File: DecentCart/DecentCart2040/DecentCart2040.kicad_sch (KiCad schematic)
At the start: 75 parts, among them J1 Micro_SD_Card, J2 Conn_02x15_Row_Letter_First, J3 SM03B-SRSS-TB, J7 Conn_01x04, J8 USB_B_Micro, J9 SM03B-SRSS-TB, Q2 DMG2305UX, SW2 SW_TACTILE, SW3 SW_TACTILE, U1 SN74LVC8T245, U2 SN74LVC8T245, U3 ATtiny1616-M, U4 NCP1117-3.3, U5 SN74LVC8T245, U6 SN74AVC4T245PW, U7 RP2040, U9 W25Q128JVS, X1 12MHz

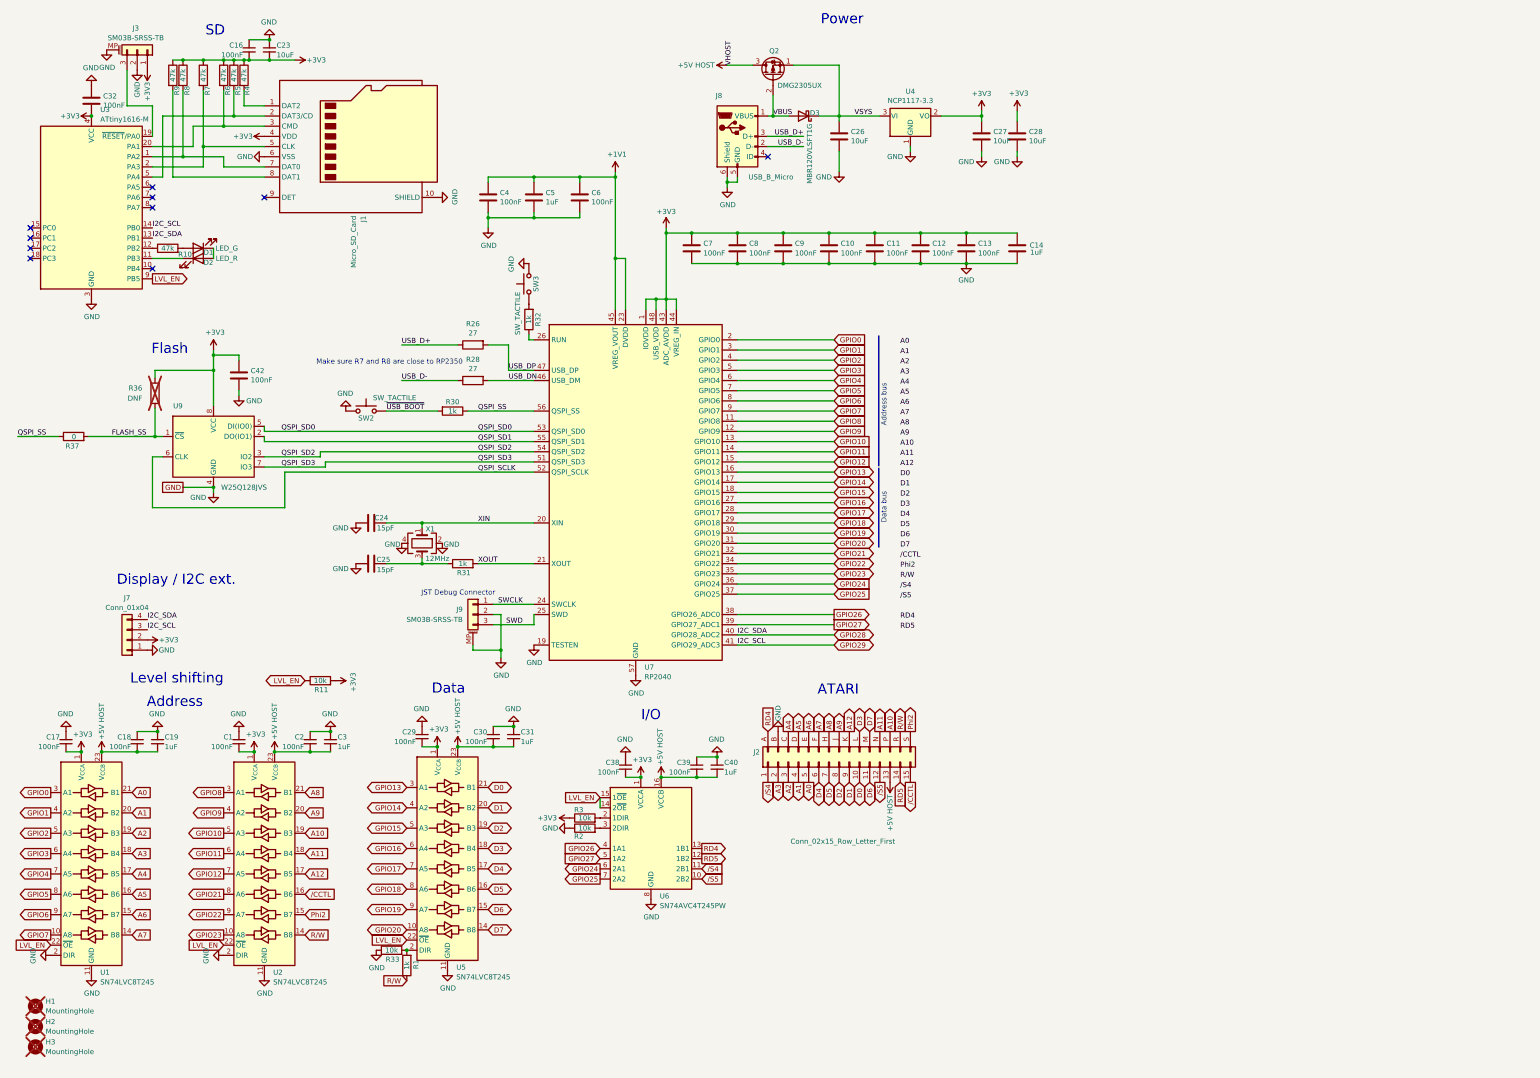
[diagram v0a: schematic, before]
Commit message: DecentCart2040 rev. 1.1
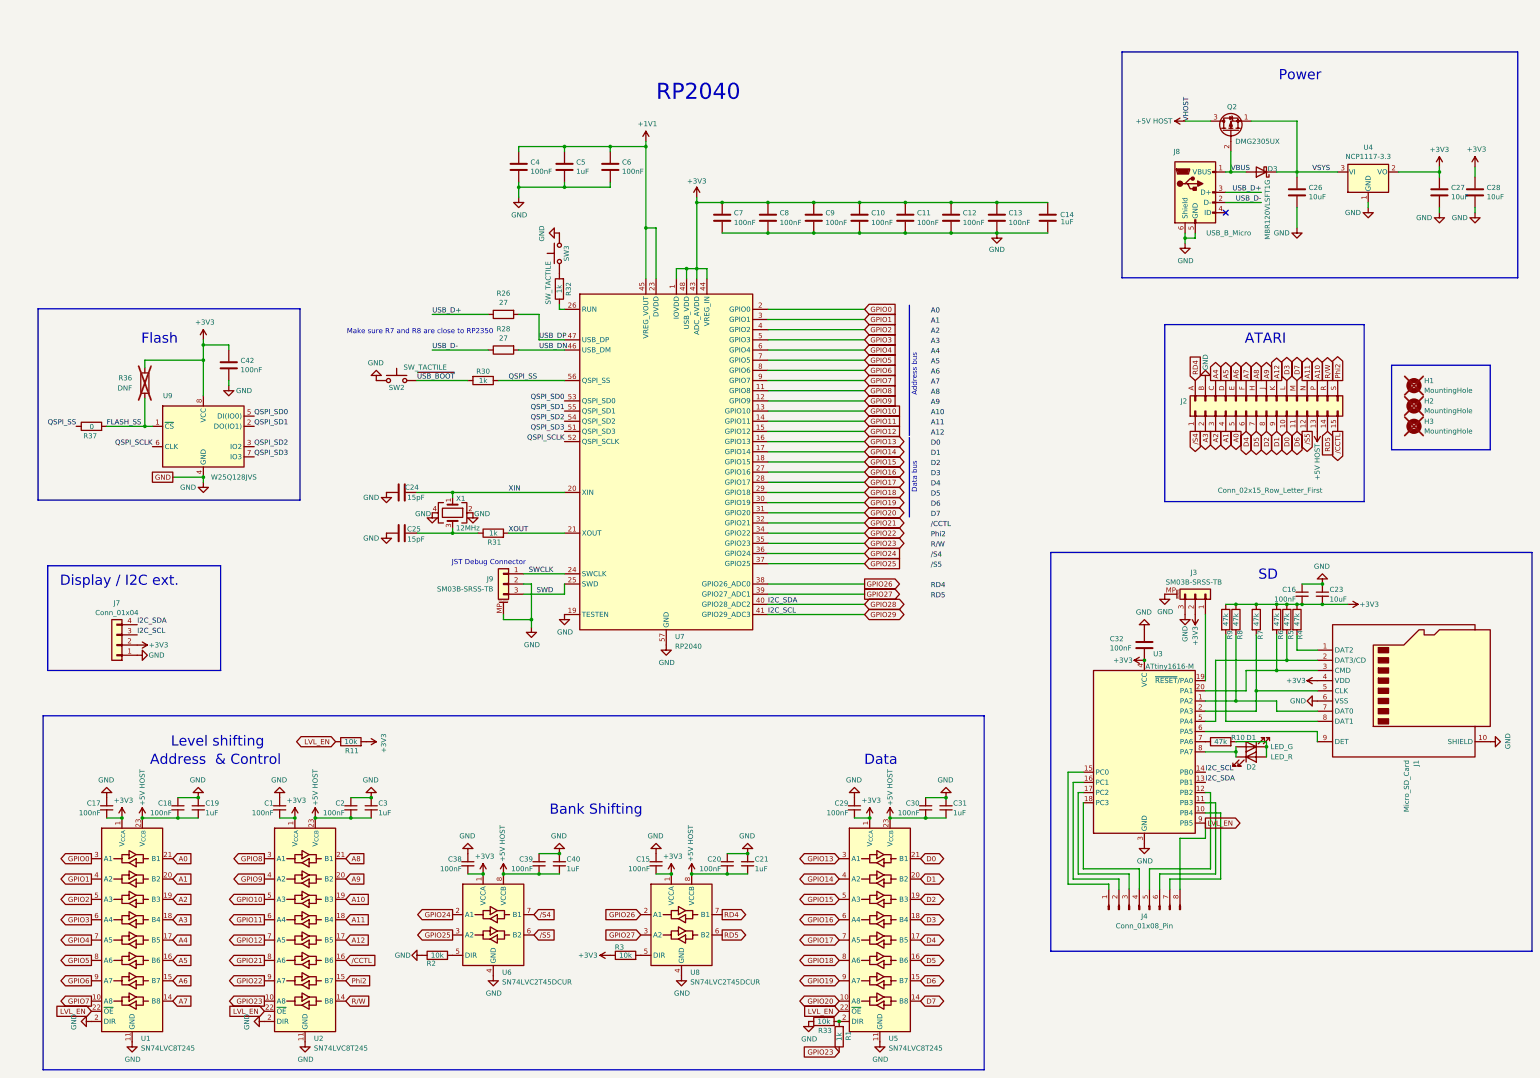
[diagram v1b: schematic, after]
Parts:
- removed U6: SN74AVC4T245PW, Package_SO:TSSOP-16_4.4x5mm_P0.65mm, symbol Logic_LevelTranslator:SN74AVC4T245PW
- added C15, C20: 100nF, Capacitor_SMD:C_0402_1005Metric, symbol Device:C_Small
- added C21: 1uF, Capacitor_SMD:C_0402_1005Metric, symbol Device:C_Small
- added J4: Conn_01x08_Pin, Connector_PinHeader_1.27mm:PinHeader_2x04_P1.27mm_Vertical, symbol Connector:Conn_01x08_Pin
- added U6, U8: SN74LVC2T45DCUR, Package_SO:VSSOP-8_2.3x2mm_P0.5mm, symbol Logic_LevelTranslator:SN74LVC2T45DCUR
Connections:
- net +3V3: now also J3.2 (Pin_2), C15.2, U6.1 (VCCA), U8.1 (VCCA); no longer J3.1 (Pin_1)
- net +5V HOST: now also C20.2, C21.2, U6.8 (VCCB), U8.8 (VCCB)
- net /S4: now also U6.7 (B1)
- net /S5: now also U6.6 (B2)
- net GND: now also J3.3 (Pin_3), C15.1, C20.1, C21.1, U6.4 (GND), U8.4 (GND); no longer J3.2 (Pin_2)
- net GPIO23: now also R1.1
- net GPIO24: now also U6.2 (A1)
- net GPIO25: now also U6.3 (A2)
- net GPIO26: now also U8.2 (A1)
- net GPIO27: now also U8.3 (A2)
- net LVL_EN: now also J4.8 (Pin_8)
- net R/W: no longer R1.1
- net RD4: now also U8.7 (B1)
- net RD5: now also U8.6 (B2)
- net at U3.10 (PB4): now also J4.7 (Pin_7)
- net at U3.11 (PB3): now also J4.6 (Pin_6); no longer D2.1 (K)
- net at U3.12 (PB2): now also J4.5 (Pin_5); no longer R10.1
- net at U3.15 (PC0): now also J4.1 (Pin_1)
- net at U3.16 (PC1): now also J4.2 (Pin_2)
- net at U3.17 (PC2): now also J4.3 (Pin_3)
- net at U3.18 (PC3): now also J4.4 (Pin_4)
- net at U3.19 (~{RESET}/PA0): now also J3.1 (Pin_1); no longer J3.3 (Pin_3)
- net at U3.6 (PA5): now also J1.9 (DET)
- net at U3.7 (PA6): now also R10.1
- net at U3.8 (PA7): now also D1.2 (A), D2.1 (K)
- net at D1.1 (K), D2.2 (A): now also R10.2
- net at R2.2: now also U6.5 (DIR)
- net at R3.2: now also U8.5 (DIR)
- no-connect marks 10 -> 1
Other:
- note added: "Address & Control"
- note added: "Bank Shifting"
- note added: "RP2040"
- note removed: "Address"
- note removed: "I/O"
- moved on the sheet: C1, C10, C11, C12, C13, C14, C16, C17, C18, C19, C2, C23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
